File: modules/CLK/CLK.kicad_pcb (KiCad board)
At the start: 2 copper layers, 160 x 100 mm, 27 parts, among them J1 CardConnector, SW1 1MS2T1B1M1QES, U1 74HCT14, U2 74HCT390, U3 74HCT390, U4 74HCT390, U5 74AHCT541, U6 555, Y1 1Mhz

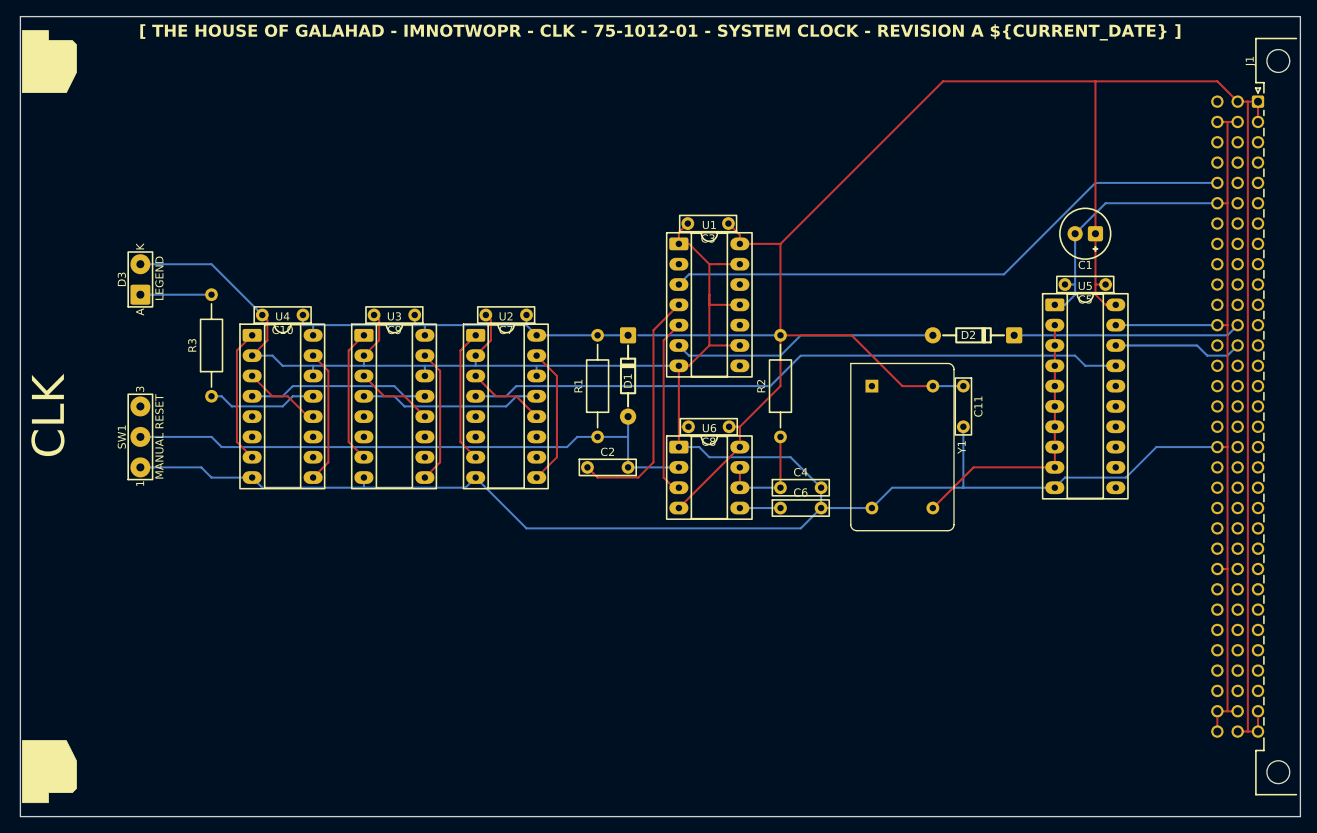
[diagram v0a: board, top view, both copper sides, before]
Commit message: added termination XXX card
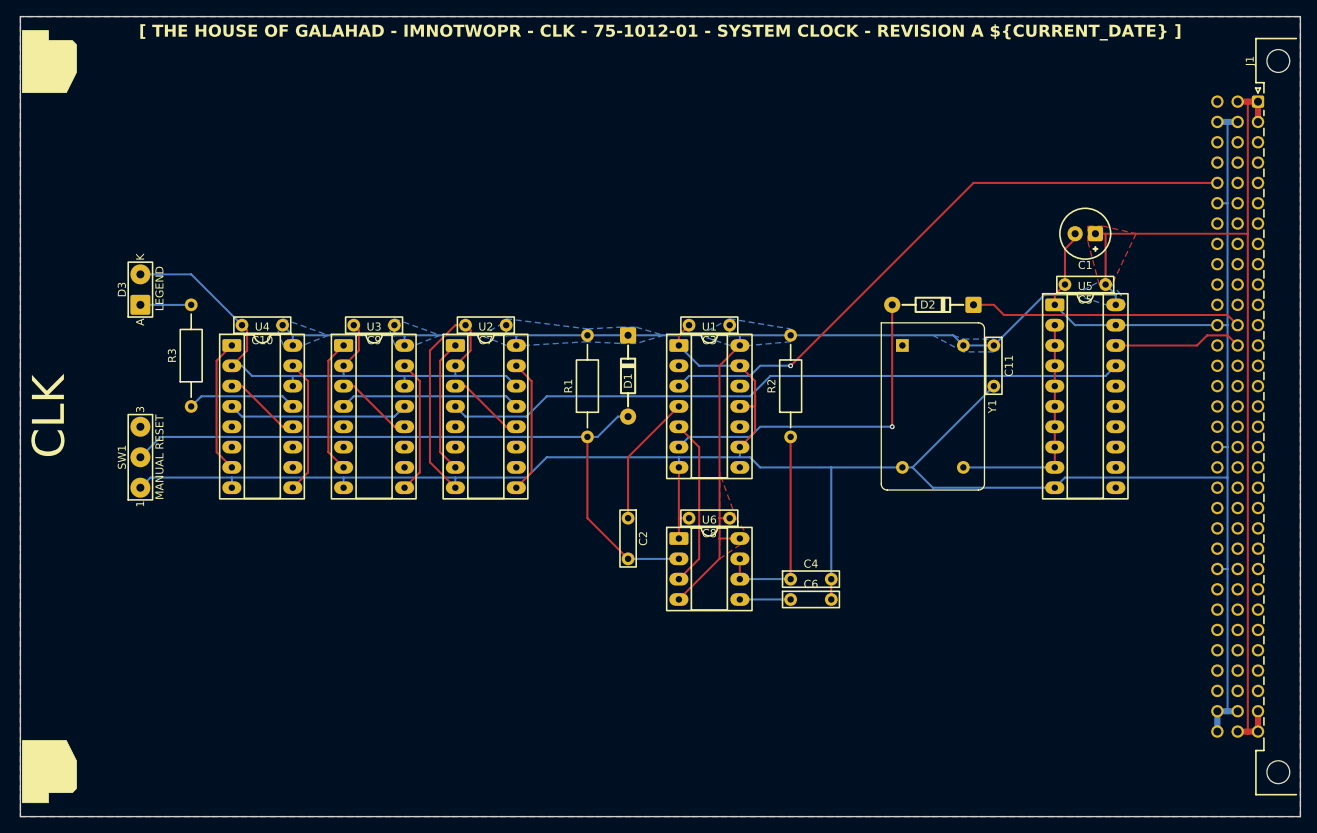
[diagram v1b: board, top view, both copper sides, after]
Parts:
- moved C3 12.7 mm to (141.1, 83.6)
- moved U1 12.7 mm to (141.1, 93.7)
- moved C4 11.5 mm to (153.8, 115.3)
- moved C6 11.5 mm to (153.8, 117.9)
- moved C8 11.4 mm to (141.1, 107.7)
- moved U6 11.4 mm to (141.1, 114.0)
- moved C2 9.25 mm to (131.0, 110.2), turned to -90 degrees
- moved C11 6.35 mm to (176.7, 88.7)
- moved Y1 6.35 mm to (165.2, 86.1)
- moved D2 6.35 mm to (169.1, 81.0)
- moved C10 2.84 mm to (85.2, 83.6)
- moved C9 2.84 mm to (99.2, 83.6)
- moved R3 2.84 mm to (76.3, 87.4)
- moved U3 2.84 mm to (99.2, 95.0)
- moved U4 2.84 mm to (85.2, 95.0)
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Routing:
- net +5V: track 325.1 -> 272.7 mm
- net GND: track 448.2 -> 430.3 mm
- net Net-(C2-Pad1): track 30.6 -> 16.6 mm
- net Net-(U6-DISCH): track 14.0 -> 26.7 mm
- net Net-(D1-A): track 74.7 -> 86.8 mm
- net Net-(D2-A): track 33.3 -> 43.0 mm, vias 0 -> 1
- net Net-(U5A-A_{0}): track 35.1 -> 29.2 mm
- net /CLK/#RESET: track 28.5 -> 34.1 mm
- net /CLK/PWROK: track 72.6 -> 77.8 mm, vias 0 -> 1
- net /CLK/PHI2_B1: track 82.6 -> 85.7 mm
- net Net-(D3-A): track 8.89 -> 6.35 mm
- net Net-(U6-CONT): track 5.08 -> 6.35 mm
- net Net-(U6-OUT): track 22.3 -> 21.2 mm
- net Net-(U2B-CP_{0}): track 17.3 -> 16.8 mm
- added copper zone on B.Cu, net +5V
- added copper zone on F.Cu, net +5V
- added copper zone on B.Cu, net GND
- added copper zone on F.Cu, net GND

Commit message: lightman cleanup; more work pending
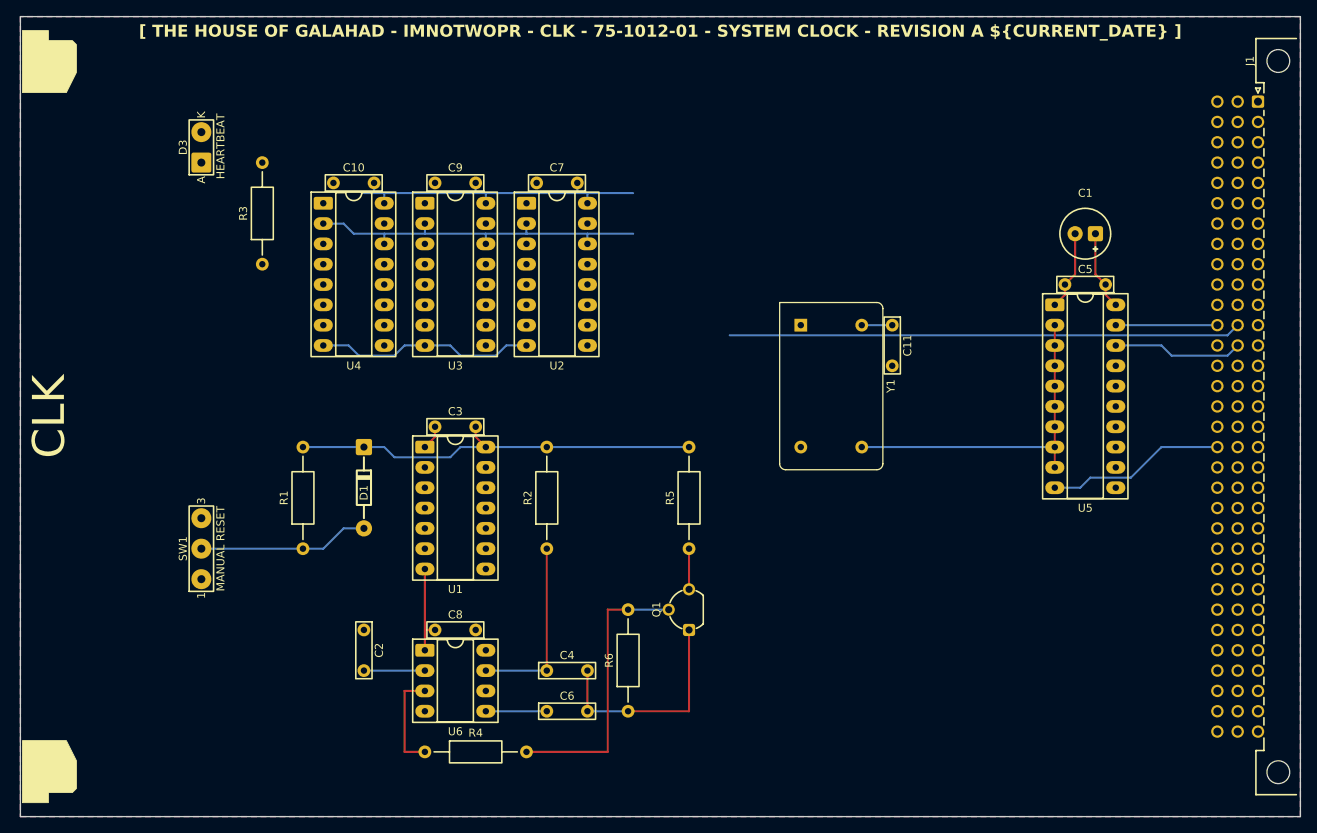
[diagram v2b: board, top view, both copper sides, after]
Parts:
- removed D2: 1N4148, FormantKO:DO-35_P400mil
- added Q1: 2N3904, IMNOTWOPR:TO-92_Wide, F.Cu at (138.6, 119.1)
- added R4: 10k, IMNOTWOPR:R_Axial_DIN0207_P400mil, F.Cu at (111.9, 136.9)
- added R5: 4k7, IMNOTWOPR:R_Axial_DIN0207_P400mil, F.Cu at (138.6, 105.2)
- added R6: 100K, IMNOTWOPR:R_Axial_DIN0207_P400mil, F.Cu at (131.0, 125.5)
- moved R1 38.2 mm to (90.3, 105.2)
- moved C2 35.9 mm to (97.9, 124.2)
- moved D1 35.9 mm to (97.9, 103.9)
- moved U6 34.7 mm to (109.4, 128.0)
- moved C8 34.7 mm to (109.4, 121.7)
- moved C3 34.2 mm to (109.4, 96.3)
- moved U1 34.2 mm to (109.4, 106.4)
- moved R2 33.5 mm to (120.8, 105.2)
- moved C6 33.5 mm to (123.3, 131.8)
- moved C4 32.6 mm to (123.3, 126.8)
- moved U4 21.1 mm to (96.7, 77.2)
- moved C10 21.1 mm to (96.7, 65.8)
- moved U3 20.5 mm to (109.4, 77.2)
- moved C9 20.5 mm to (109.4, 65.8)
- moved R3 19.9 mm to (85.2, 69.6)
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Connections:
- U1 pad 5: Net-(U6-OUT) -> GND
- U1 pad 6: Net-(D2-A) -> unconnected-(U1-Pad6)
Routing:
- net GND: track 430.3 -> 160.6 mm
- net +5V: track 272.7 -> 107.4 mm
- net /CLK/PHI2_B1: track 85.7 -> 0.00 mm
- net /CLK/PWROK: track 77.8 -> 0.00 mm, vias 1 -> 0
- net Net-(D1-A): track 86.8 -> 29.0 mm
- net Net-(D2-A): track 43.0 -> 0.00 mm, vias 1 -> 0
- net Net-(Q1-B): track 0.00 -> 35.6 mm
- net /CLK/#RESET: track 34.1 -> 69.1 mm
- net Net-(U2B-Q_{0}): track 22.6 -> 0.00 mm
- net Net-(U3B-Q_{0}): track 22.6 -> 0.00 mm
- net Net-(U4B-CP_{0}): track 16.8 -> 0.00 mm
- net Net-(U4A-CP_{0}): track 16.8 -> 0.00 mm
- net Net-(U3B-CP_{0}): track 16.8 -> 0.00 mm
- net Net-(U3A-CP_{0}): track 16.8 -> 0.00 mm
- net Net-(U2B-CP_{0}): track 16.8 -> 0.00 mm
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- removed copper zone on B.Cu, net +5V
- removed copper zone on F.Cu, net +5V
